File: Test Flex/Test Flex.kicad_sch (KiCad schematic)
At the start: 10 parts, among them J1 Conn_01x02, J2 Conn_01x02, U1 ADG728

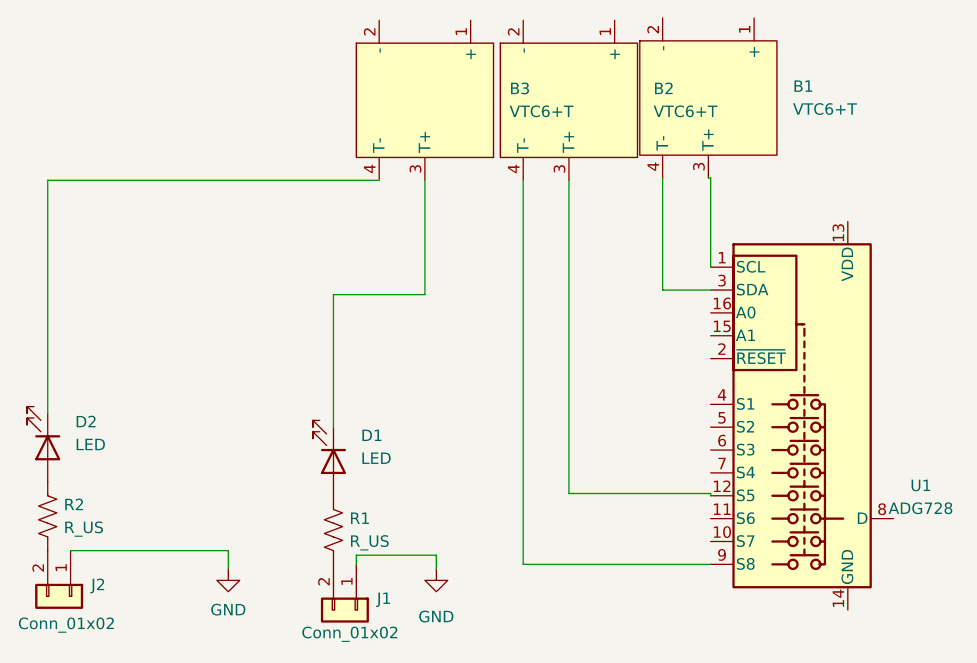
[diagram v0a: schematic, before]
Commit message: Everybody is in their general local!
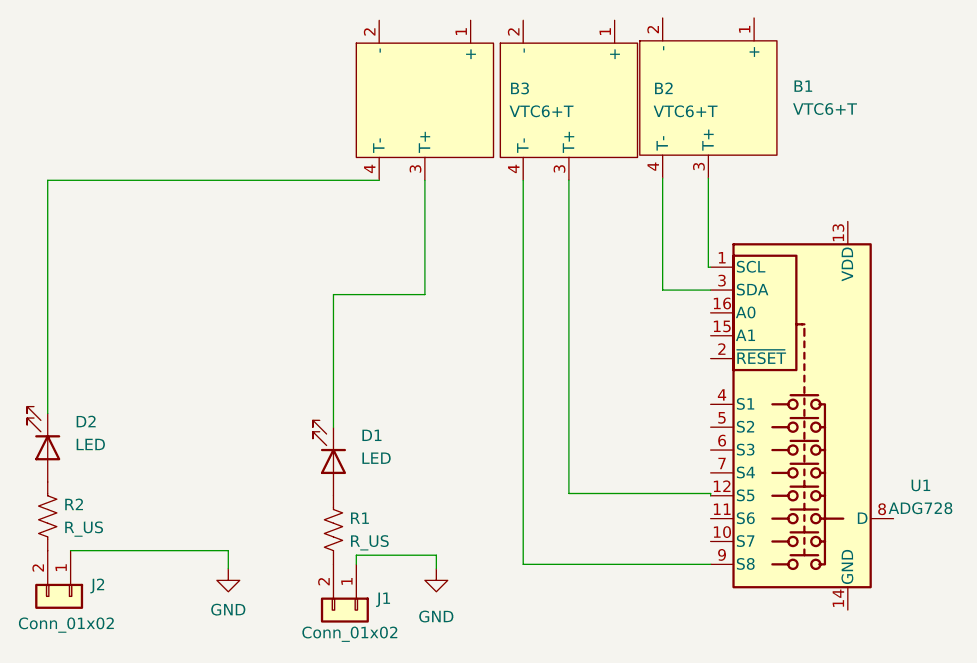
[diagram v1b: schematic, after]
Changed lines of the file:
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@@
     (stroke (width 0) (type default))
   )
-  (wire (pts (xy 189.484 56.388) (xy 189.484 46.482))
+  (wire (pts (xy 189.23 56.388) (xy 189.23 46.482))
+    (stroke (width 0) (type default))
+  )
+  (wire (pts (xy 189.23 56.388) (xy 189.484 56.388))
     (stroke (width 0) (type default))
   )
@@
     (stroke (width 0) (type default))
   )
-  (wire (pts (xy 189.484 46.482) (xy 189.23 46.482))
-    (stroke (width 0) (type default))
-  )
